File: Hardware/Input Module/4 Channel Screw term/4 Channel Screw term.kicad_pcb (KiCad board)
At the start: 2 copper layers, 43.4 x 31.5 mm, 22 parts, among them J1 Screw_Terminal_01x06, J2 Screw_Terminal_01x06, J5 Conn_01x12_Male, U1 LTV-847S, U2 74HC7014

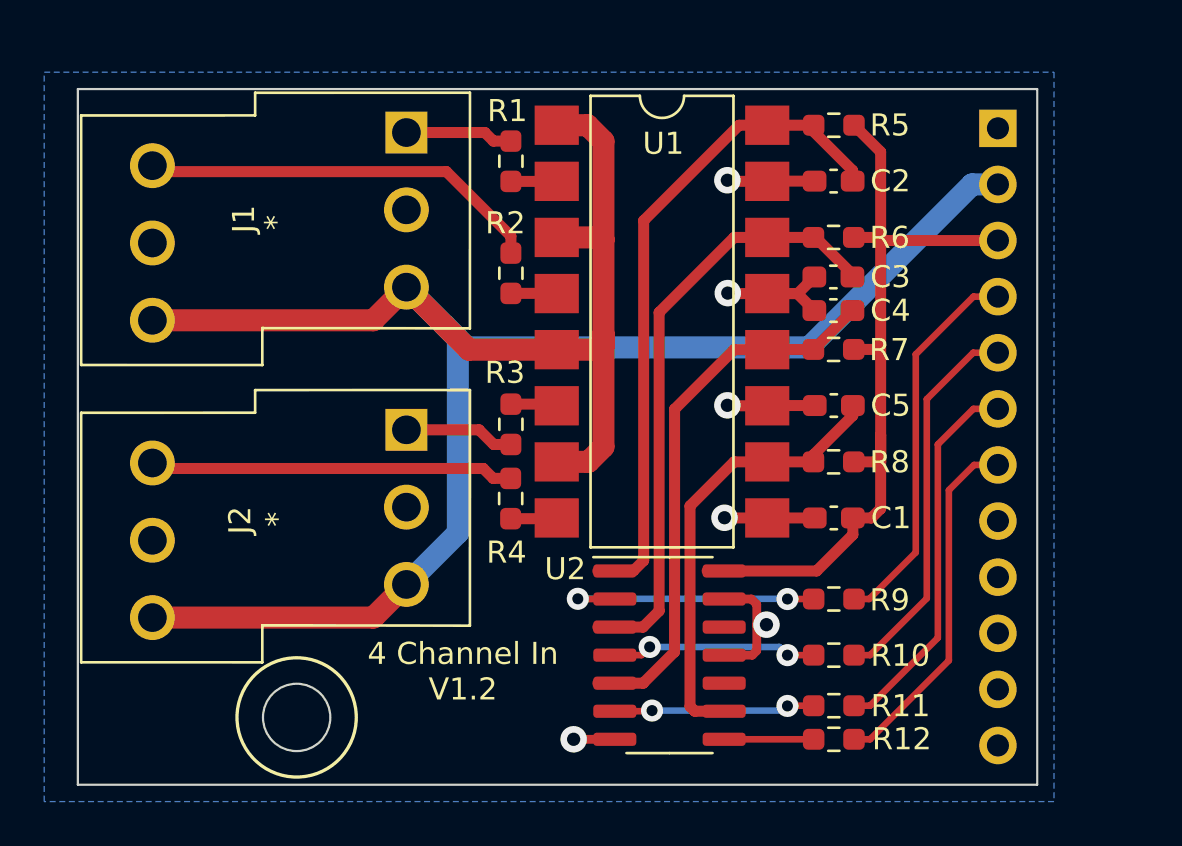
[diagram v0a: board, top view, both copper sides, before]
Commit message: Random changes
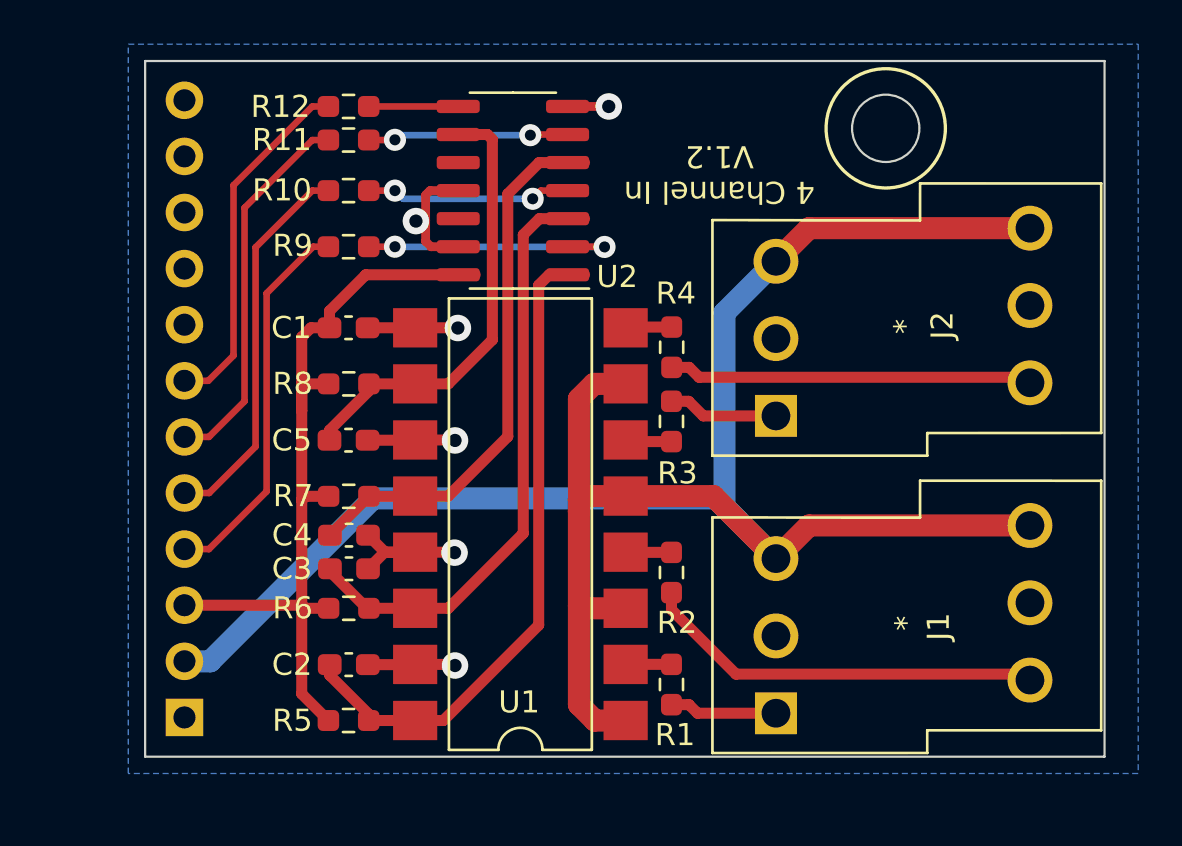
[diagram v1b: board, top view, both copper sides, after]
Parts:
- moved J1 46.1 mm to (186.9, 88.5), turned to 90 degrees
- moved J5 45.5 mm to (148.6, 90.2), turned to 0 degrees
- moved J2 39.9 mm to (186.9, 75.0), turned to 90 degrees
- moved R12 36.1 mm to (156.0, 62.5), turned to 0 degrees
- moved R5 34.8 mm to (156.0, 90.3), turned to 0 degrees
- moved R11 33.7 mm to (156.0, 64.0), turned to 0 degrees
- moved C2 31.0 mm to (156.0, 87.8), turned to 0 degrees
- moved R10 30.4 mm to (156.0, 66.3), turned to 0 degrees
- moved R6 27.6 mm to (156.0, 85.2), turned to 0 degrees
- moved R9 27.1 mm to (156.0, 68.9), turned to 0 degrees
- moved C3 25.6 mm to (156.0, 83.4), turned to 0 degrees
- moved R1 24.8 mm to (170.6, 88.7), turned to -90 degrees
- moved C4 24.2 mm to (156.0, 81.9), turned to 0 degrees
- moved C1 23.6 mm to (156.0, 72.5), turned to 0 degrees
- moved R7 22.9 mm to (156.0, 80.2), turned to 0 degrees
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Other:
- outline, holes or cut-outs redrawn
